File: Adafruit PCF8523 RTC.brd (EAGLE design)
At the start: 21.6 x 25.4 mm, 16 parts, among them IC1 RTC_PCF8523T, Q1 32.768

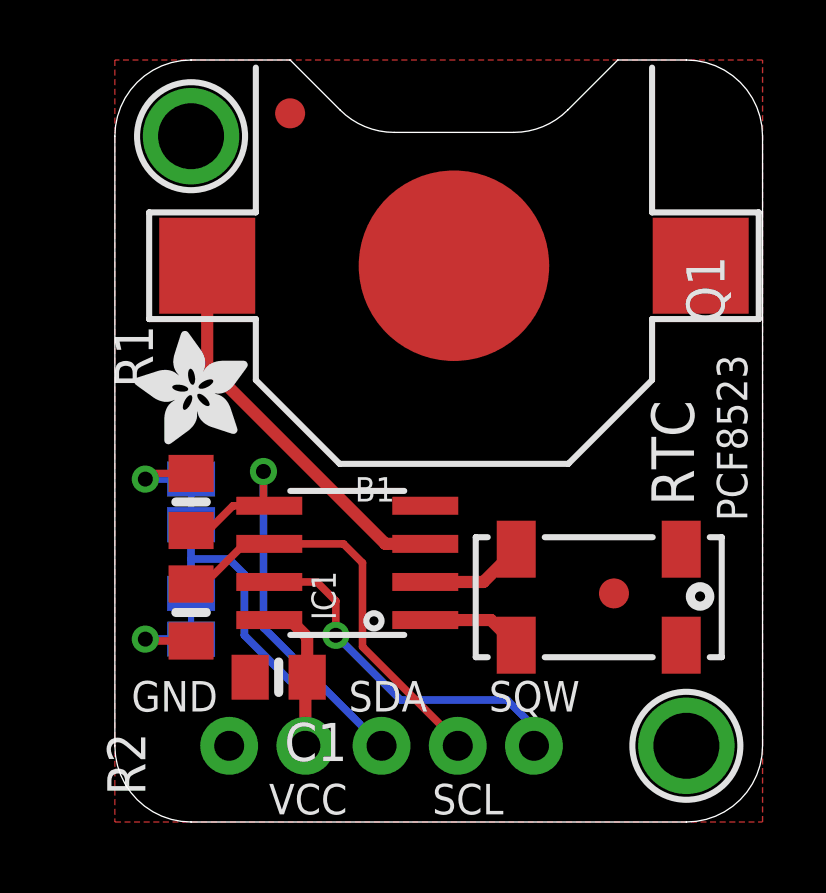
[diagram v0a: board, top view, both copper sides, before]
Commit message: https://github.com/adafruit/Adafruit-PCF8523-RTC-Breakout-PCB/issues/1
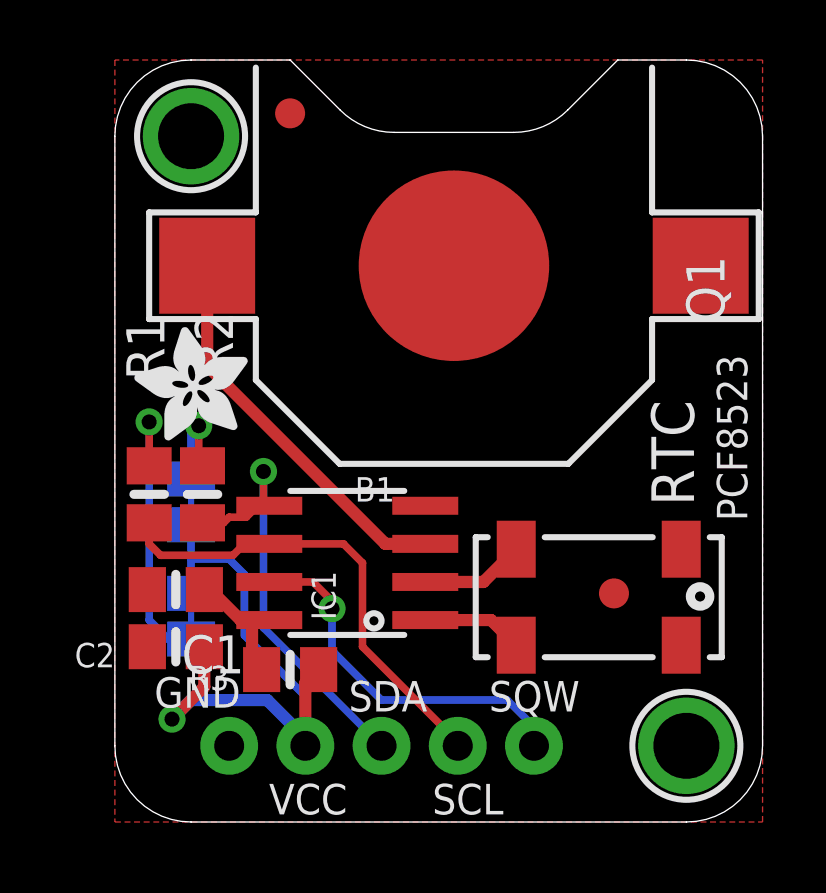
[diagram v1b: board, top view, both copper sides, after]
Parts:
- added C2: 10uF, microbuilder:0805-NO
- added R3: 1K, microbuilder:0805-NO
- C1: value 0.1uF -> 10uF
- moved C1 4.50 mm to (2.03, 7.75)
- moved R2 4.18 mm to (1.14, 10.9), turned to 270 degrees
- moved R1 0.46 mm to (2.92, 10.9)
- moved U$2 0.13 mm to (4.45, 12.7)
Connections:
- new net N$3: C1.1, IC1.8, R3.2
- net GND: now also C2.2
- net VCC: now also C2.1, R3.1; no longer C1.1, IC1.8
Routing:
- net N$1: track 3.07 -> 9.73 mm
- net VCC: track 16.0 -> 21.9 mm, vias 0 -> 1
- net N$3: track 0.00 -> 4.37 mm
- net SCL: track 13.9 -> 15.8 mm
- net SDA: track 14.9 -> 14.3 mm
